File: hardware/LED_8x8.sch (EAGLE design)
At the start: 3 parts

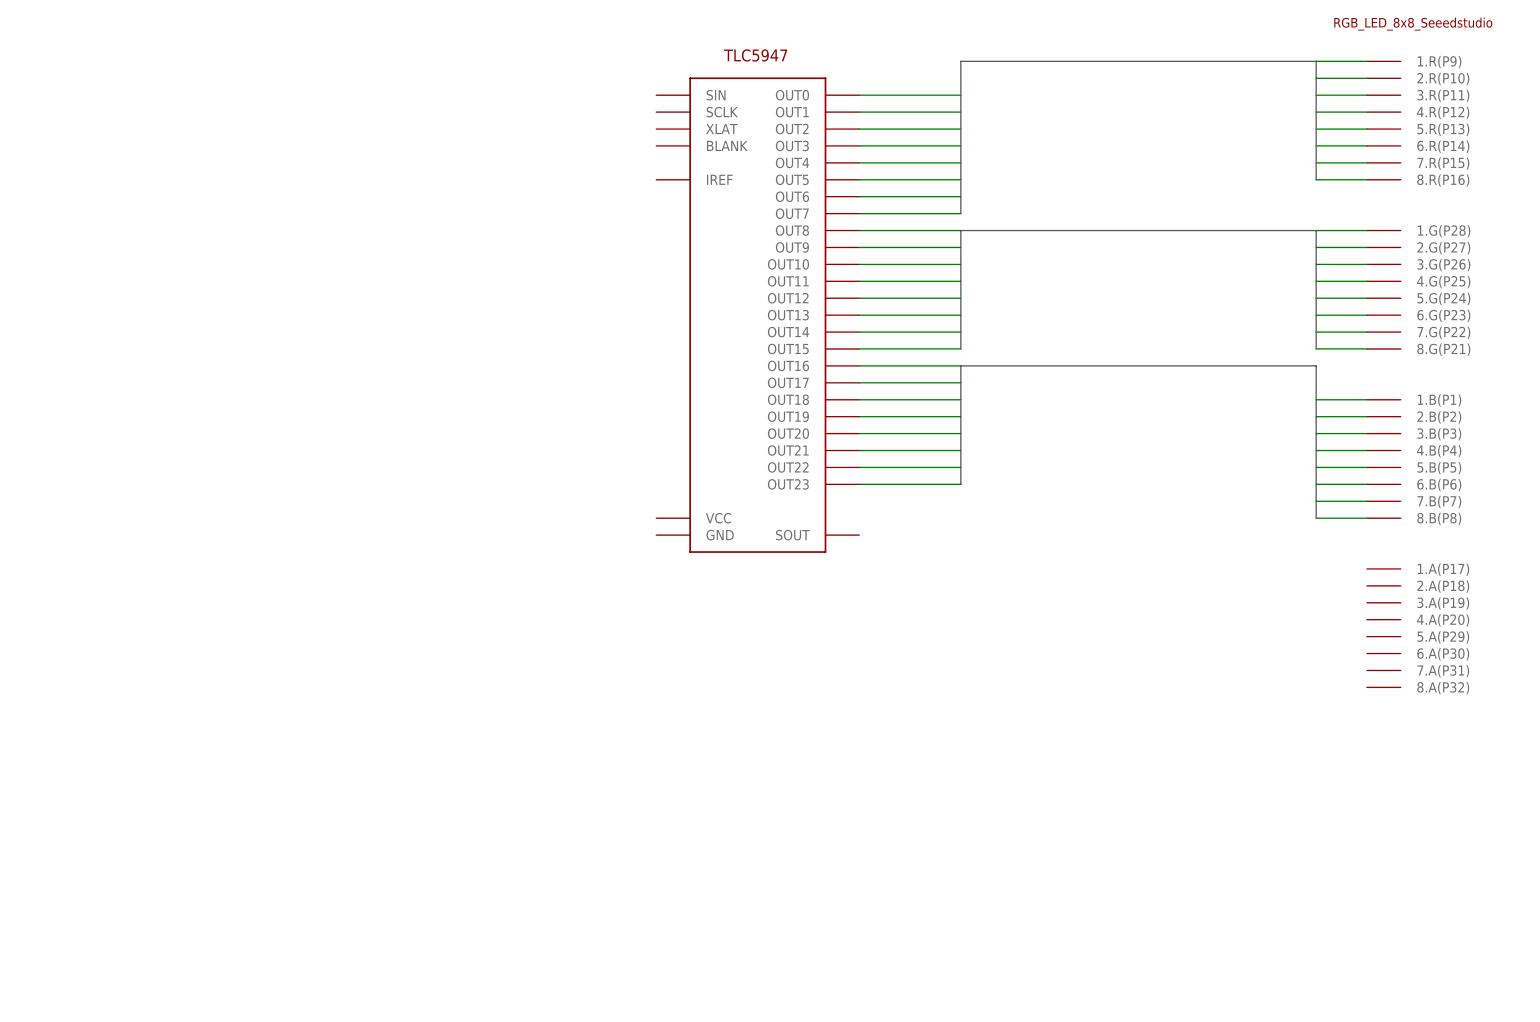
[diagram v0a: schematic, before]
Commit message: progress, bitches
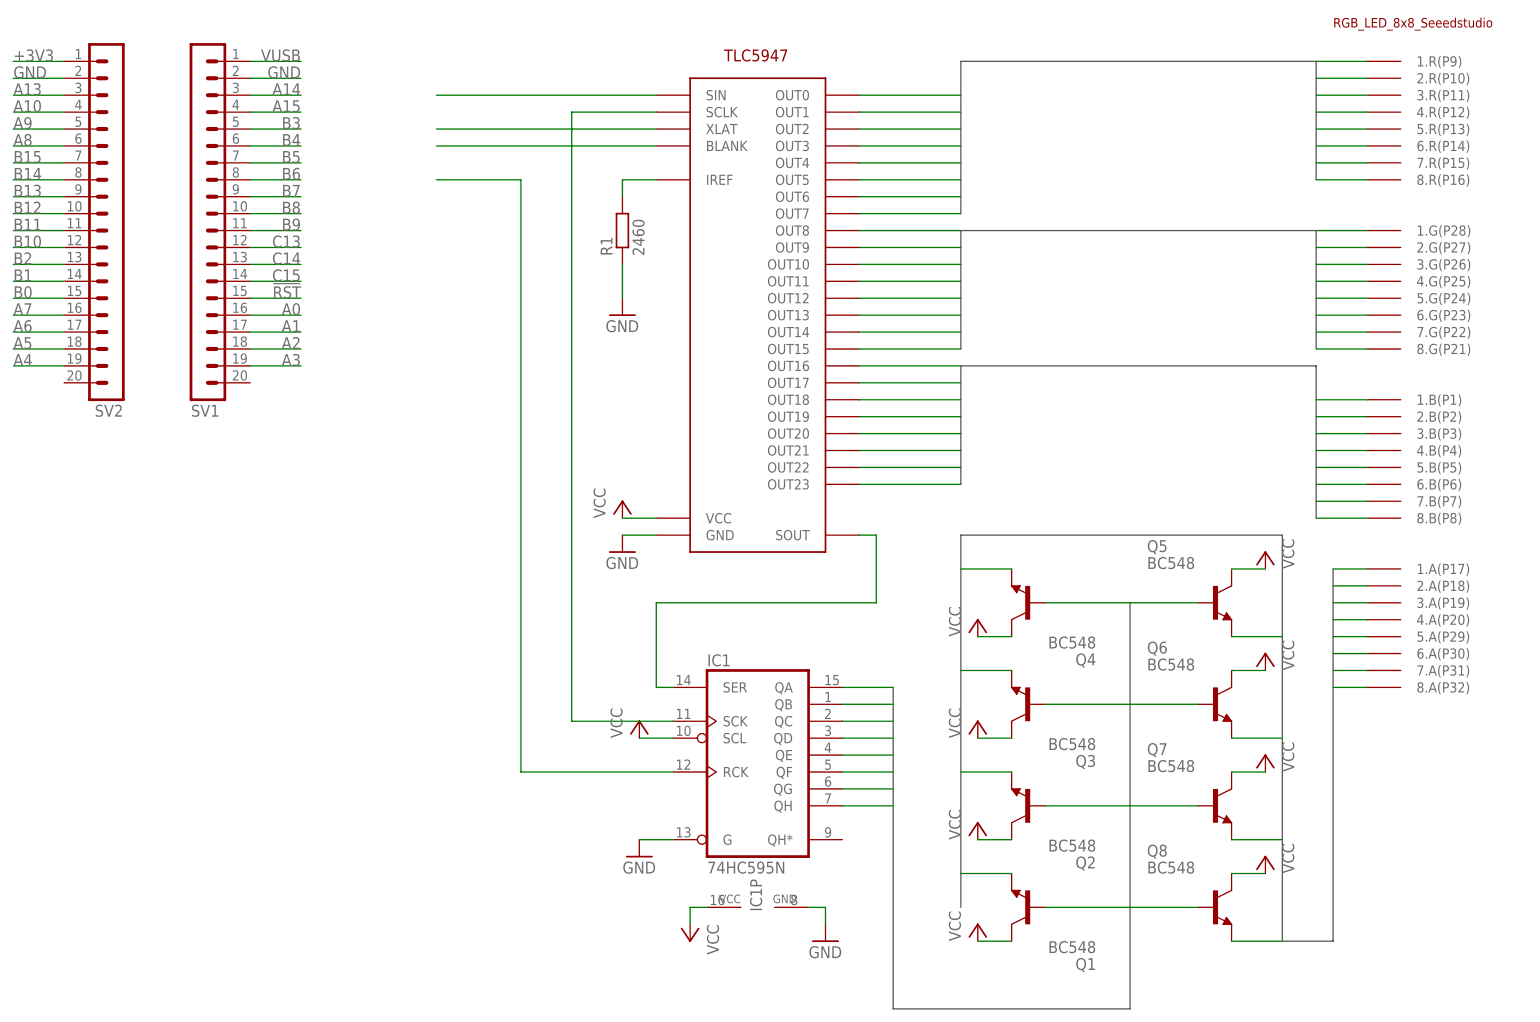
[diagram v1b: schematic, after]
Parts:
- removed U$2: SHACKLOGO, shack:SHACKLOGO
- added IC1: 74HC595N, 74xx-eu:74HC595N
- added Q1, Q2, Q3, Q4, Q5, Q6, Q7, Q8: BC548, transistor-npn:BC548
- added R1: 2460, rcl:R-EU_R0603
- added SV1, SV2: (no value), con-lstb:MA20-1
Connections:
- new net !RST: SV1.15
- new net +3V3: SV2.1
- new net A0: SV1.16
- new net A1: SV1.17
- new net A10: SV2.4
- new net A13: SV2.3
- new net A14: SV1.3
- new net A15: SV1.4
- new net A2: SV1.18
- new net A3: SV1.19
- new net A4: SV2.19
- new net A5: SV2.18
- new net A6: SV2.17
- new net A7: SV2.16
- new net A8: SV2.6
- new net A9: SV2.5
- new net B0: SV2.15
- new net B1: SV2.14
- new net B10: SV2.12
- new net B11: SV2.11
- new net B12: SV2.10
- new net B13: SV2.9
- new net B14: SV2.8
- new net B15: SV2.7
- new net B2: SV2.13
- new net B3: SV1.5
- new net B4: SV1.6
- new net B5: SV1.7
- new net B6: SV1.8
- new net B7: SV1.9
- new net B8: SV1.10
- new net B9: SV1.11
- new net C13: SV1.12
- new net C14: SV1.13
- new net C15: SV1.14
- new net GND: IC1A.G, IC1P.GND, R1.1, SV1.2, SV2.2, U$1.GND
- new net N$1: IC1A.SER, U$1.SOUT
- new net N$2: IC1A.SCK, U$1.SCLK
- new net N$3: IC1A.RCK
- new net N$4: U$1.SIN
- new net N$5: U$1.XLAT
- new net N$6: U$1.BLANK
- new net N$7: R1.2, U$1.IREF
- new net POWERA1: Q1.E, U$3.1.A(P17)
- new net POWERA2: Q2.E, U$3.2.A(P18)
- new net POWERA3: Q3.E, U$3.3.A(P19)
- new net POWERA4: Q4.E, U$3.4.A(P20)
- new net POWERA5: Q5.E, U$3.5.A(P29)
- new net POWERA6: Q6.E, U$3.6.A(P30)
- new net POWERA7: Q7.E, U$3.7.A(P31)
- new net POWERA8: Q8.E, U$3.8.A(P32)
- new net SHIFTA1: IC1A.QA, Q1.B
- new net SHIFTA2: IC1A.QB, Q2.B
- new net SHIFTA3: IC1A.QC, Q3.B
- new net SHIFTA4: IC1A.QD, Q4.B
- new net SHIFTA5: IC1A.QE, Q5.B
- new net SHIFTA6: IC1A.QF, Q6.B
- new net SHIFTA7: IC1A.QG, Q7.B
- new net SHIFTA8: IC1A.QH, Q8.B
- new net VCC: IC1A.SCL, IC1P.VCC, Q1.C, Q2.C, Q3.C, Q4.C, Q5.C, Q6.C, Q7.C, Q8.C, U$1.VCC
- new net VUSB: SV1.1
